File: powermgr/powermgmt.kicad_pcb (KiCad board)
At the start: 2 copper layers, 83.8 x 40.1 mm, 58 parts, among them IC1 74HC4094_RevA_23Aug2012, IC2 AP24x1, IC3 AP24x1, IC4 AP24x1, IC5 AP24x1, IC6 AP24x1, IC7 AP24x1, IC8 AP24x1, IC9 AP24x1, J1 CONN_01X06, J2 CONN_01X06, J3 CONN_01X02, J4 CONN_01X02, P1 CONN_01X16

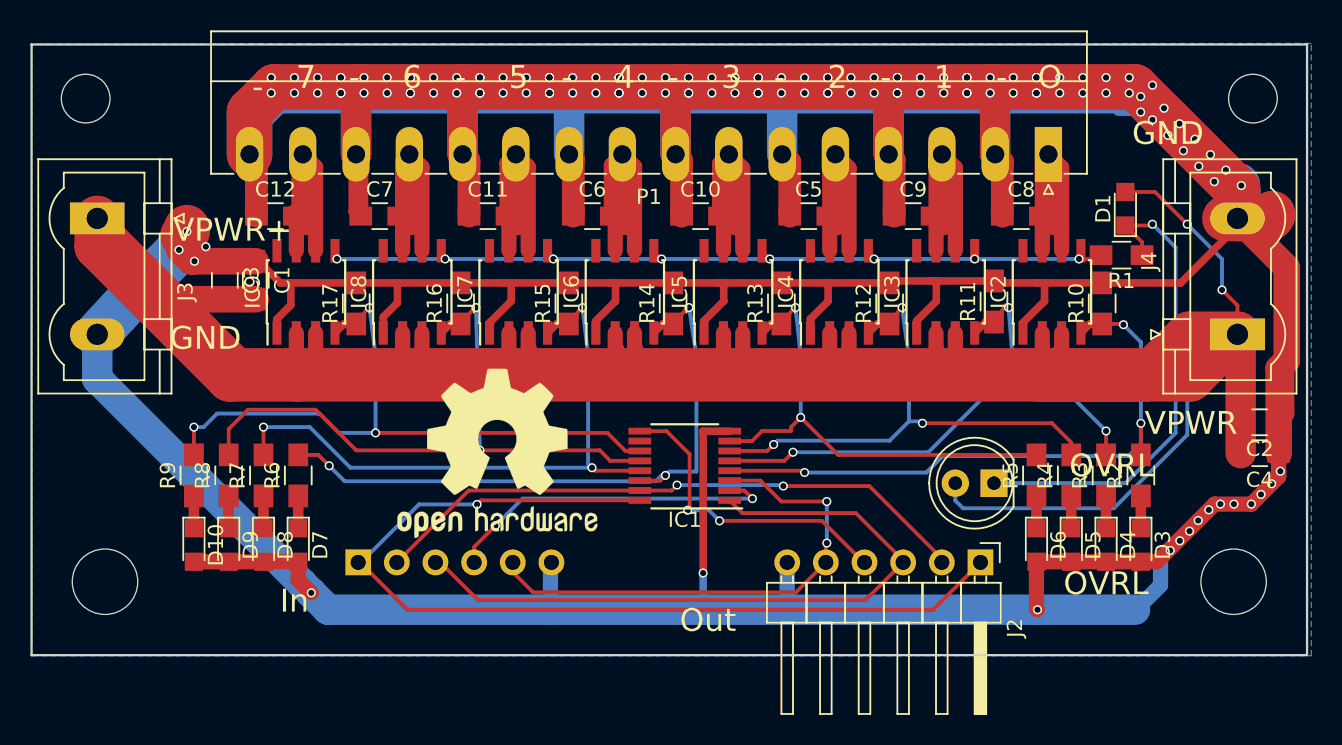
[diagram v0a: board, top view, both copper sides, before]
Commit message: fixups and text
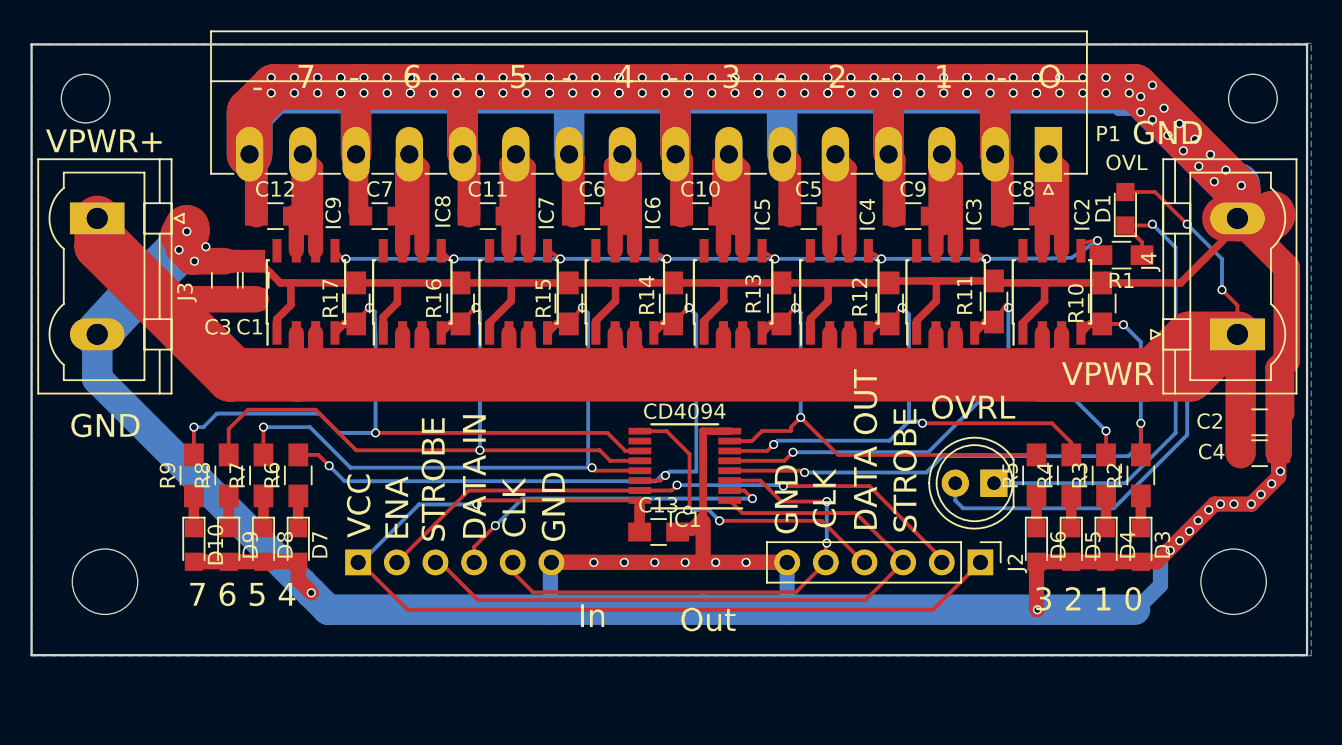
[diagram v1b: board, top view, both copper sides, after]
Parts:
- added C13: 100n, Capacitors_SMD:C_0805_HandSoldering, F.Cu at (57.2, 46.8)
- IC1: value 74HC4094_RevA_23Aug2012 -> CD4094
- J1: value CONN_01X06 -> IN; footprint Pin_Headers:Pin_Header_Angled_1x06_Pitch2.54mm -> Pin_Headers:Pin_Header_Straight_1x06_Pitch2.54mm
- J2: value CONN_01X06 -> OUT; footprint Pin_Headers:Pin_Header_Angled_1x06_Pitch2.54mm -> Pin_Headers:Pin_Header_Straight_1x06_Pitch2.54mm
- P1: value CONN_01X16 -> PWR_OUT
- REF***: moved to B.Cu
- moved REF*** 45.6 mm to (92.1, 37.9), turned to 180 degrees
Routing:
- net GND: track 714.8 -> 745.3 mm, vias 130 -> 135
- net OVERLOAD: track 54.6 -> 59.8 mm
- net VCC: track 63.7 -> 65.8 mm
- net /Power out/out_pwr1: track 18.1 -> 19.0 mm
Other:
- board text added: "2A per out, 2.1-2.5 triggers current limit OVRL will lit if any outputs gets overloaded Outputs will have resistance if off (cap disch. func.) Controlling: CLK DATA in -> STROBE low -> ENABLE high ENA low will shut off all outputs"
- board text added: "3 2 1 0"
- board text added: "7 6 5 4"
- board text added: "CLK"
- board text added: "DATA IN"
- board text added: "DATA OUT"
- board text added: "ENA"
- board text added: "OVL"
- board text added: "STROBE"
- board text added: "VCC"
- board text added: "https://github.com/XANi/ee/tree/master/powermgr"
